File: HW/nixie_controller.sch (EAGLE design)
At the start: 201 parts, among them IC1 INA138, IC10 LD1117S33TR, IC11 74HC595D, IC2 LM386M-1, IC3 7812TV, IC4 DG408DYTSSOP-16, IC5 OPA317DBV, IC6 OPA317DBV, IC7 OPA340U, IC8 OPA340U, IC9 NE555D, J1 POWER_JACKPTH_LOCK, Q10 DMP3099L-7, Q11 MMBT3906, Q2 CMPT5551, Q3 CMPT5551, Q4 CMPT5551, Q5 FMMT558QTA, Q6 CMPT5551, Q7 MMBT3906, Q8 CMPT5551, Q9 CMPT5551, T1 MMBT3904, T2 MMBT3904

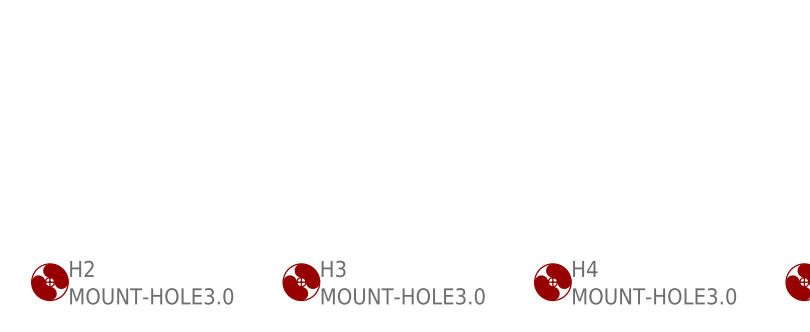
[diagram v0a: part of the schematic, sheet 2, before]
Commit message: Aktualizace aktuální verze desky , nákup a pod.
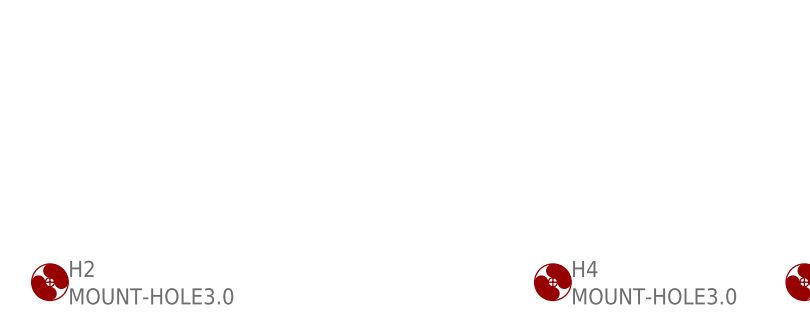
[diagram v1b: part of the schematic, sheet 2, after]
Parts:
- removed H3: MOUNT-HOLE3.0, holes:MOUNT-HOLE3.0
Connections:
- net EXT_MCU: now also JP1.1; no longer JP1.2
- net GND: now also JP1.2; no longer JP1.1
